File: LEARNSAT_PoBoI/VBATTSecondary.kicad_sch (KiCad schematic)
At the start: 17 parts, among them Q701 SI7164DP-T1-GE3, Q702 SI5418DU-T1-GE3, U701 INA219AIDCNR, U702 LTC4231IUD-2#TRPBF

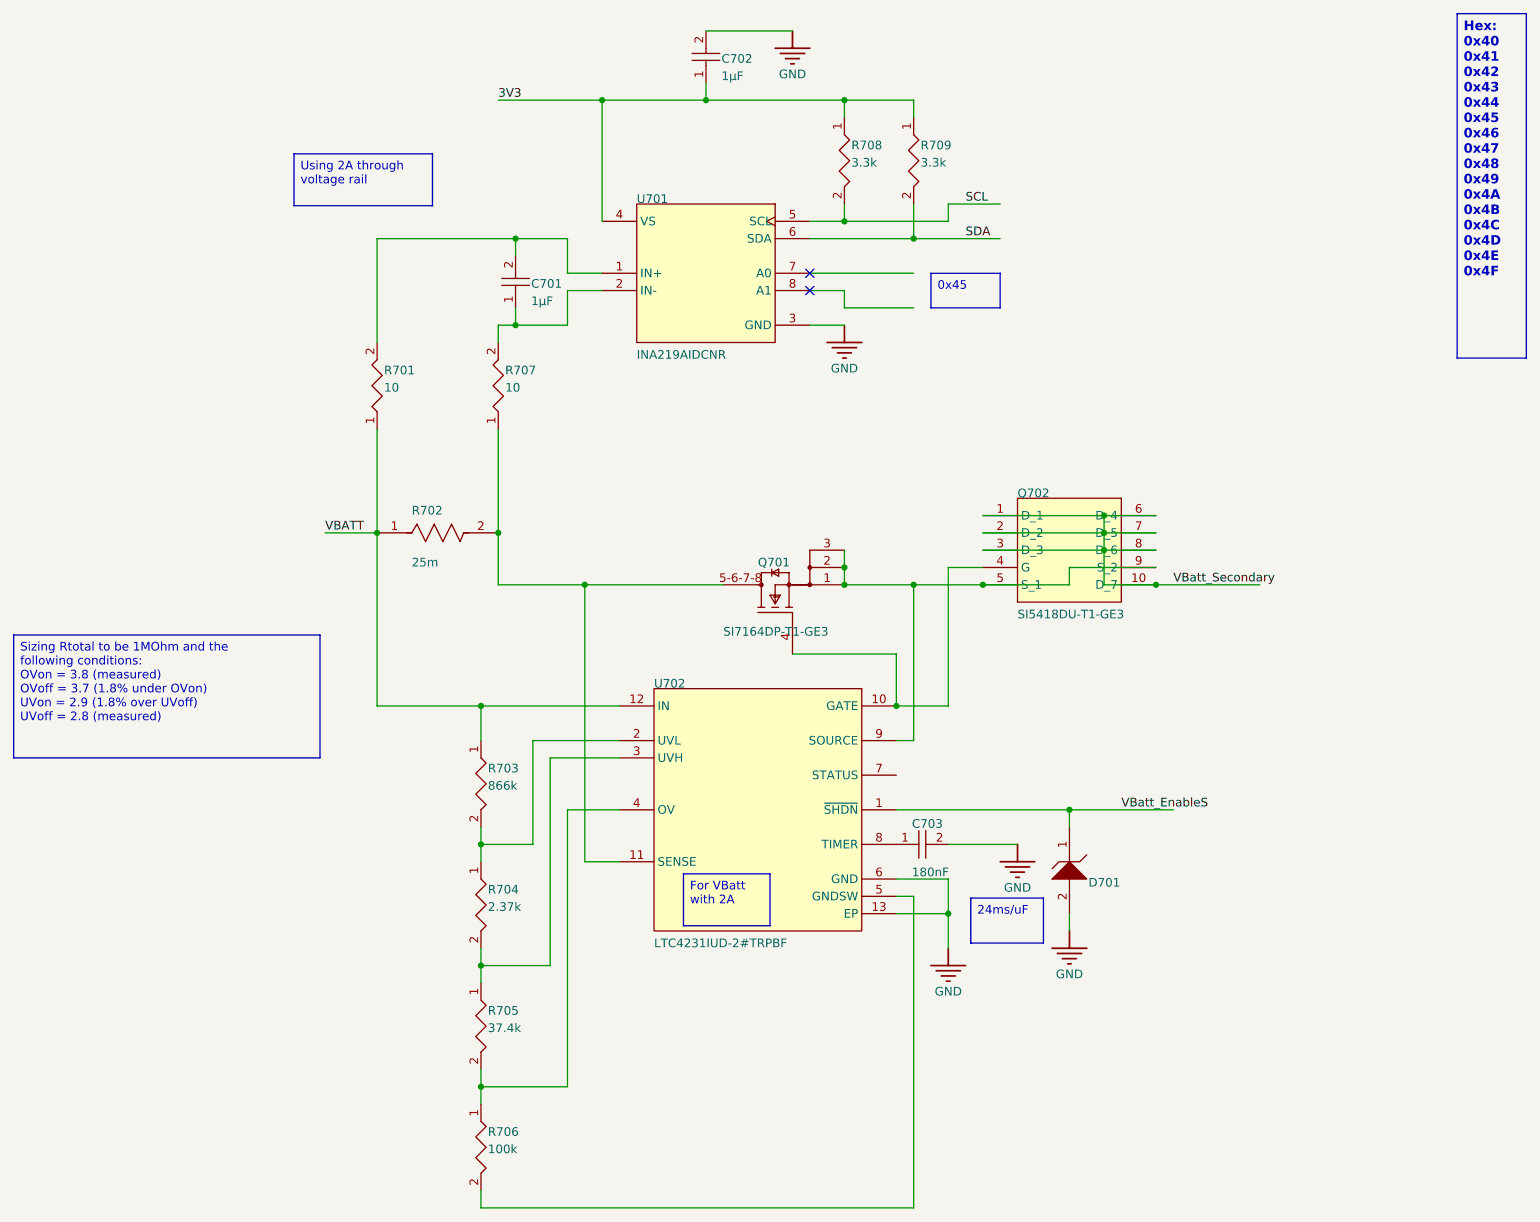
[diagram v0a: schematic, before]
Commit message: Add files via upload
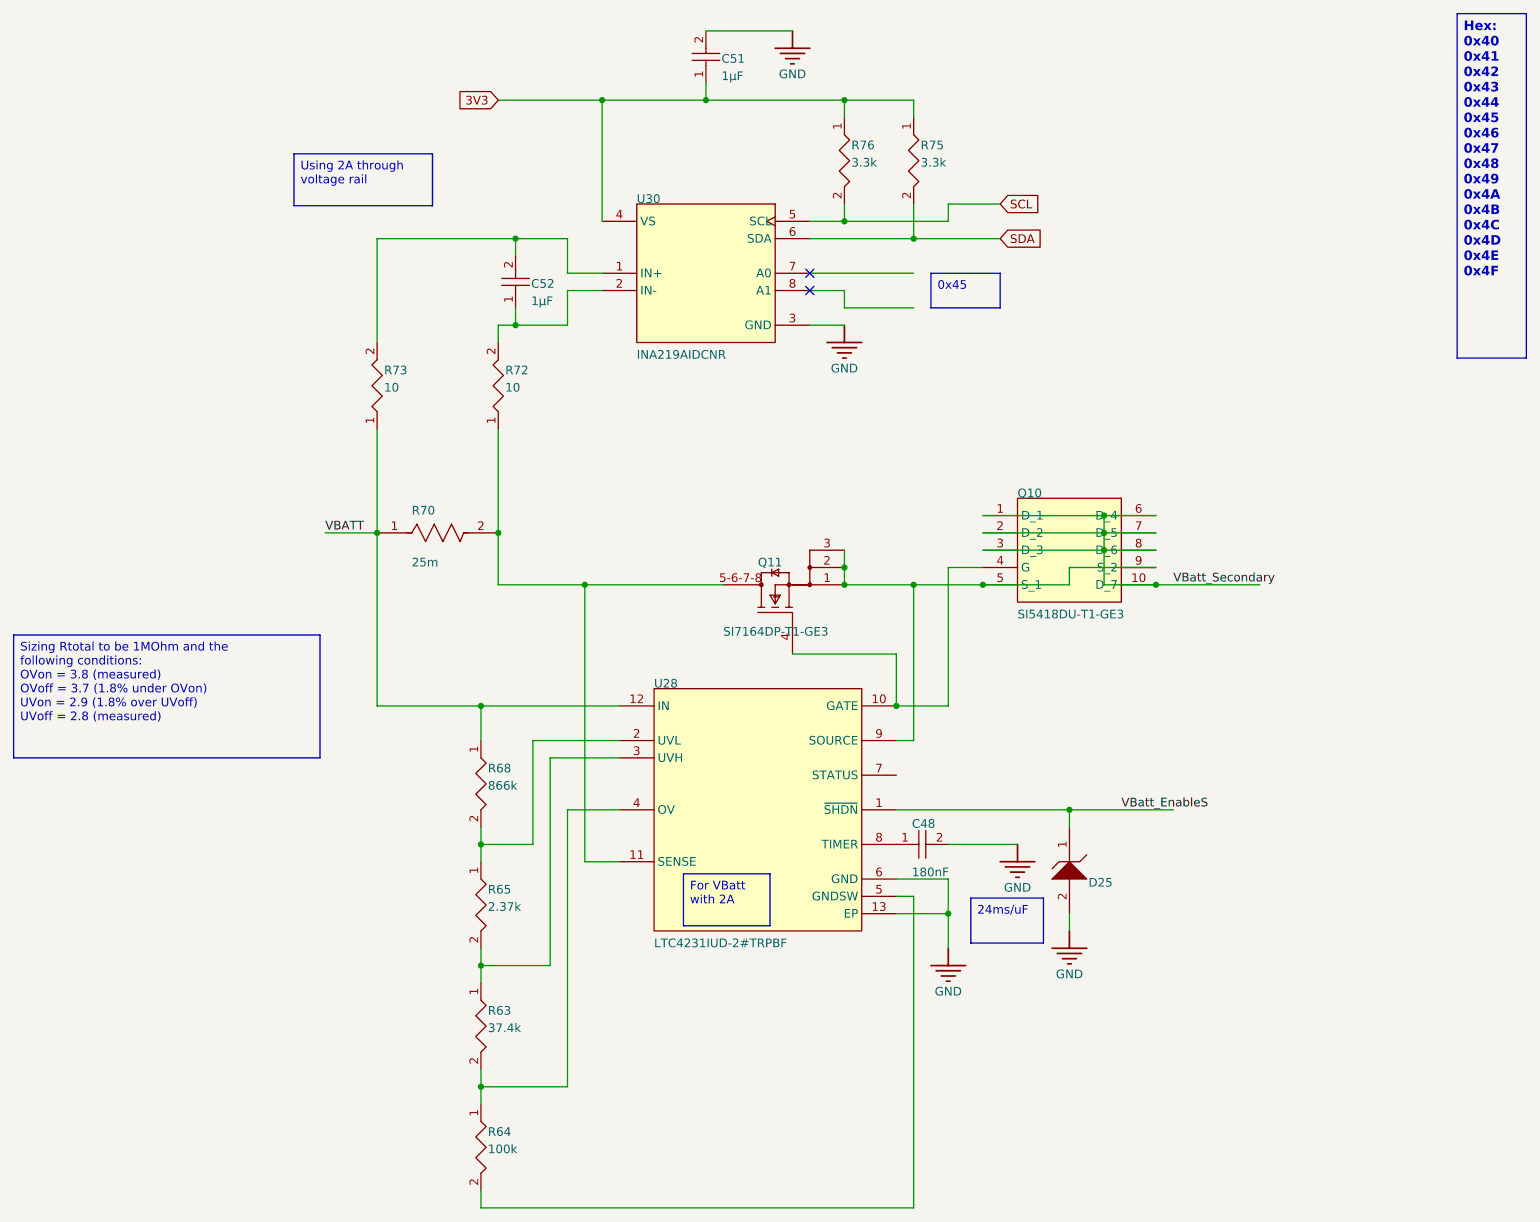
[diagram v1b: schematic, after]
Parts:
- C48: renamed from C703; footprint Capacitor_SMD:C_0805_2012Metric -> FP-C0805C-DN-IPC_A
- C51: renamed from C702; footprint Capacitor_SMD:C_0603_1608Metric -> CAPC1608X90X35ML15T15
- C52: renamed from C701; footprint Capacitor_SMD:C_0603_1608Metric -> CAPC1608X90X40LL10T20
- D25: renamed from D701; footprint Diode_SMD:D_SOD-323 -> ONSC-SOD-323-2-477-02_V
- Q10: renamed from Q702; footprint Package_SO:Vishay_PowerPAK_1212-8_Single -> SI5418DU-T1-GE3-Footprint-1
- Q11: renamed from Q701; footprint Package_SO:Vishay_PowerPAK_1212-8_Single -> Vishay_S17-0173-SINGLE_MFG
- R63: renamed from R705; footprint Resistor_SMD:R_0603_1608Metric -> FP-CR0603-IPC_A
- R64: renamed from R706; footprint Resistor_SMD:R_0402_1005Metric -> RESC1005X40X25ML05T05
- R65: renamed from R704; footprint Resistor_SMD:R_0402_1005Metric -> RESC0402(1005)_L
- R68: renamed from R703; footprint Resistor_SMD:R_0603_1608Metric -> RESC0603X26X15NL03T05
- R70: renamed from R702; footprint Resistor_SMD:R_1206_3216Metric -> FP-CSR1206-IPC_C
- R72: renamed from R707; footprint Resistor_SMD:R_0402_1005Metric -> RESC0402(1005)_L
- R73: renamed from R701; footprint Resistor_SMD:R_0402_1005Metric -> RESC0402(1005)_L
- R75: renamed from R709; footprint Resistor_SMD:R_1210_3225Metric -> FP-CRCW1210-e3-IPC_C
- R76: renamed from R708; footprint Resistor_SMD:R_1210_3225Metric -> FP-CRCW1210-e3-IPC_C
- U28: renamed from U702; footprint LTC4231IUD-2_TRPBF:QFN50P300X300X80-13N -> FP-UD-12-05-08-1855-IPC_A
- U30: renamed from U701; footprint INA219AIDCNR:SOT65P280X145-8N -> FP-DCN0008A-IPC_A

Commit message: Added footprints
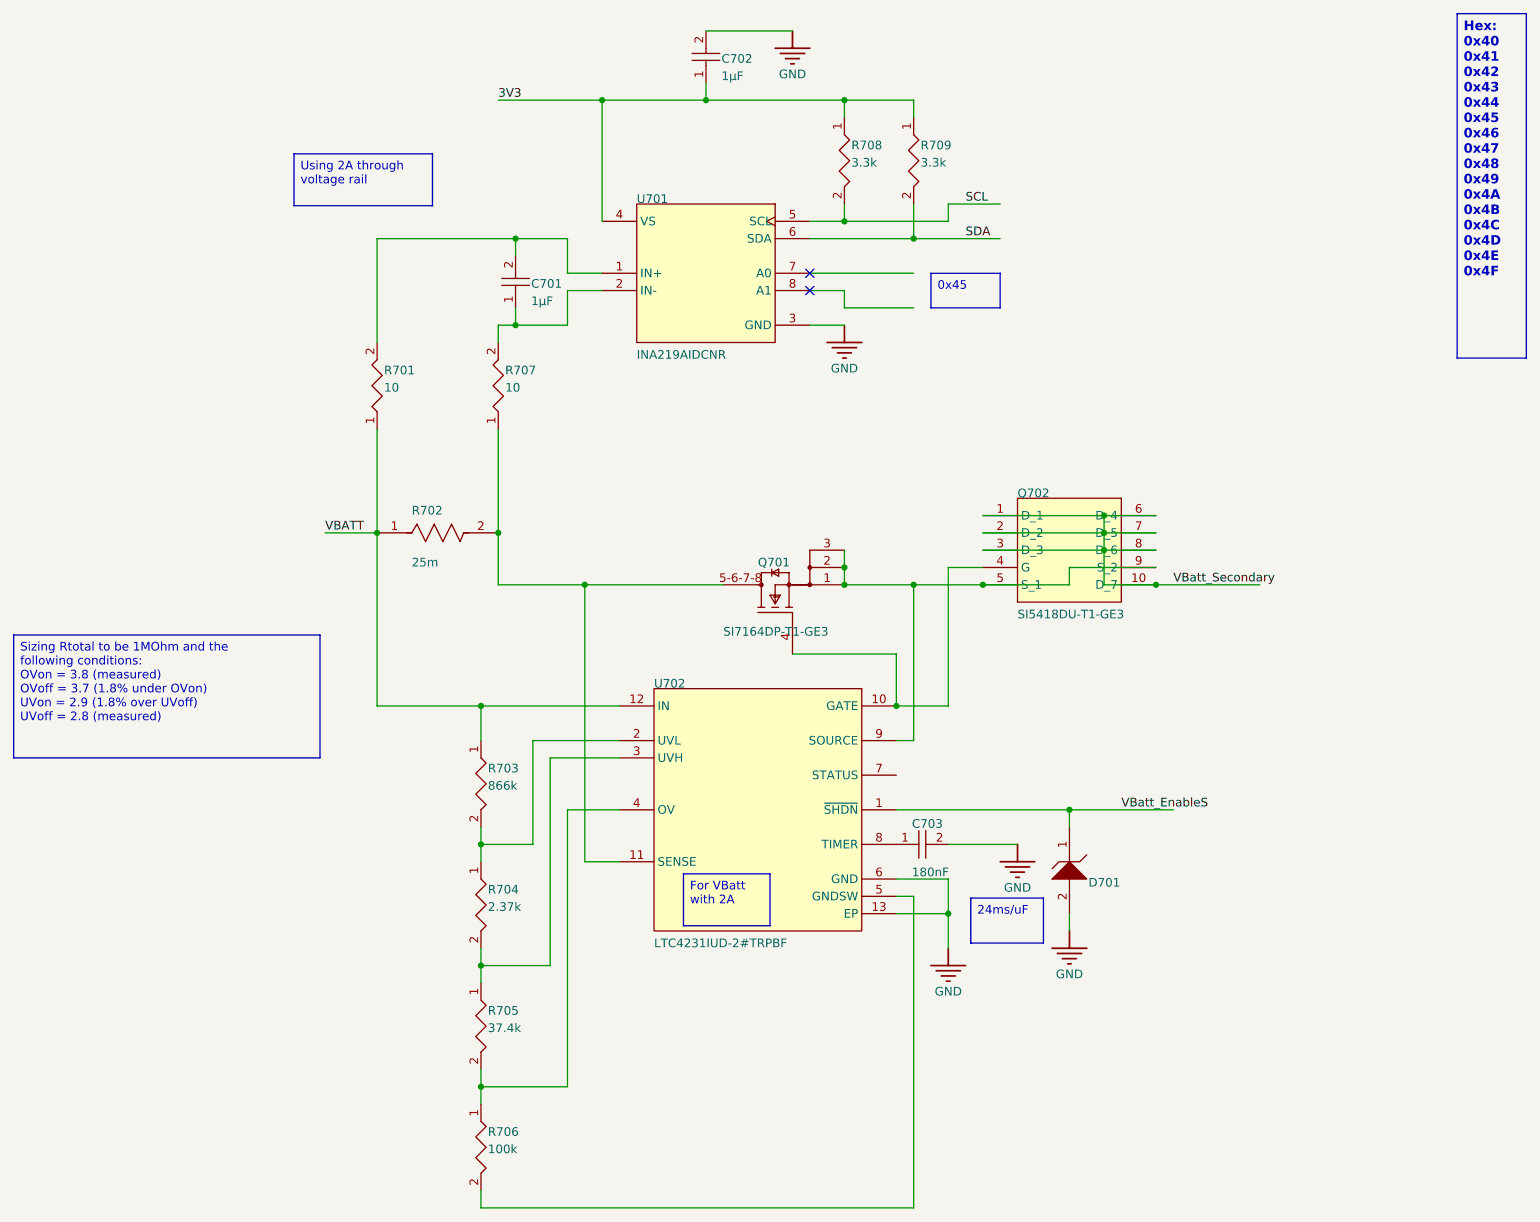
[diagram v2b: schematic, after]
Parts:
- C701: renamed from C52; footprint CAPC1608X90X40LL10T20 -> Capacitor_SMD:C_0603_1608Metric
- C702: renamed from C51; footprint CAPC1608X90X35ML15T15 -> Capacitor_SMD:C_0603_1608Metric
- C703: renamed from C48; footprint FP-C0805C-DN-IPC_A -> Capacitor_SMD:C_0805_2012Metric
- D701: renamed from D25; footprint ONSC-SOD-323-2-477-02_V -> Diode_SMD:D_SOD-323
- Q701: renamed from Q11; footprint Vishay_S17-0173-SINGLE_MFG -> Package_SO:Vishay_PowerPAK_1212-8_Single
- Q702: renamed from Q10; footprint SI5418DU-T1-GE3-Footprint-1 -> Package_SO:Vishay_PowerPAK_1212-8_Single
- R701: renamed from R73; footprint RESC0402(1005)_L -> Resistor_SMD:R_0402_1005Metric
- R702: renamed from R70; footprint FP-CSR1206-IPC_C -> Resistor_SMD:R_1206_3216Metric
- R703: renamed from R68; footprint RESC0603X26X15NL03T05 -> Resistor_SMD:R_0603_1608Metric
- R704: renamed from R65; footprint RESC0402(1005)_L -> Resistor_SMD:R_0402_1005Metric
- R705: renamed from R63; footprint FP-CR0603-IPC_A -> Resistor_SMD:R_0603_1608Metric
- R706: renamed from R64; footprint RESC1005X40X25ML05T05 -> Resistor_SMD:R_0402_1005Metric
- R707: renamed from R72; footprint RESC0402(1005)_L -> Resistor_SMD:R_0402_1005Metric
- R708: renamed from R76; footprint FP-CRCW1210-e3-IPC_C -> Resistor_SMD:R_1210_3225Metric
- R709: renamed from R75; footprint FP-CRCW1210-e3-IPC_C -> Resistor_SMD:R_1210_3225Metric
- U701: renamed from U30; footprint FP-DCN0008A-IPC_A -> INA219AIDCNR:SOT65P280X145-8N
- U702: renamed from U28; footprint FP-UD-12-05-08-1855-IPC_A -> LTC4231IUD-2_TRPBF:QFN50P300X300X80-13N
